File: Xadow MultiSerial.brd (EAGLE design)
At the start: 25.4 x 20.3 mm, 19 parts, among them J1 12p 0.5mm bottom contact, J2 12p 0.5mm bottom contact, J3 12p 0.5mm bottom contact, J4 12p 0.5mm bottom contact, U1 SC16IS752, X1 CTS_32X25_SMD

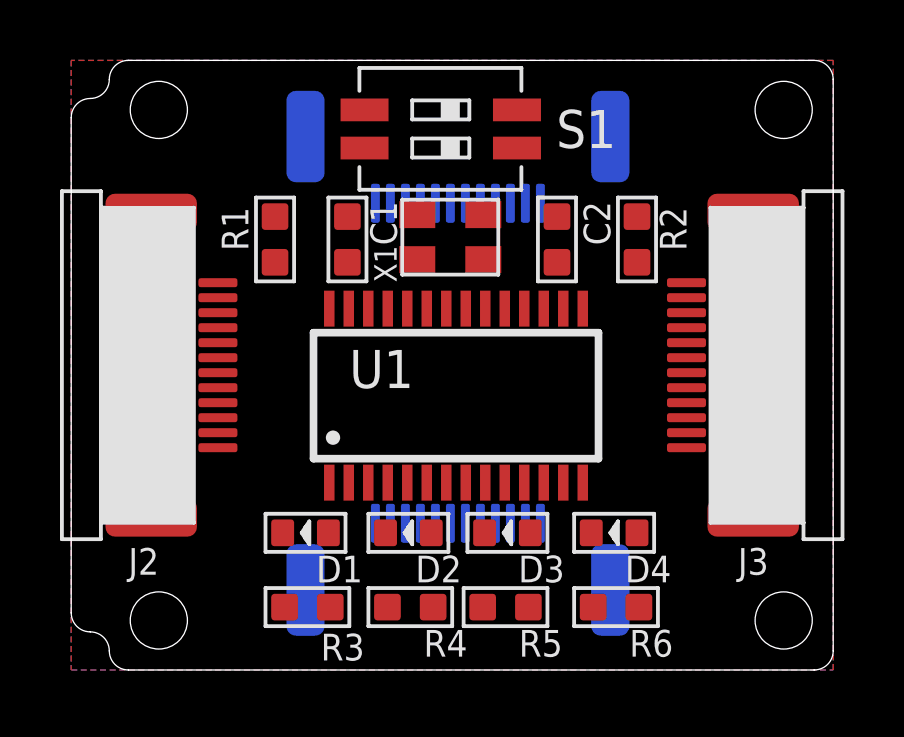
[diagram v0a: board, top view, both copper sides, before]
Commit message: Added level shifter MOSFETs
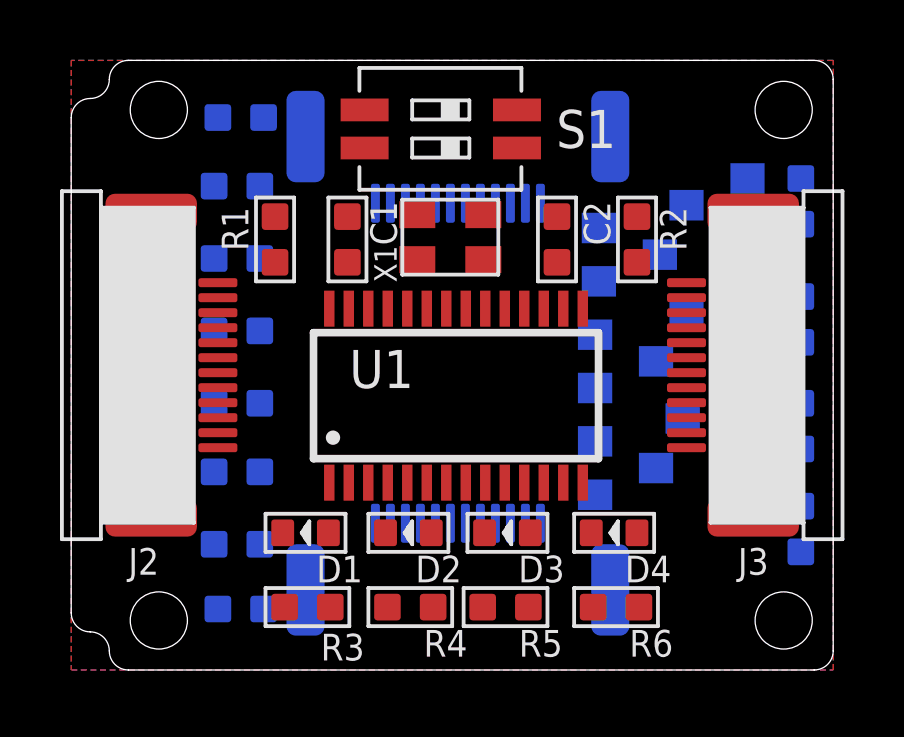
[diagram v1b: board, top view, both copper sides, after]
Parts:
- added Q1, Q2, Q3, Q4, Q5, Q6: MOSFET-N-044020001, OPL:SOT23
- added R10, R11, R12, R13, R14, R15, R16, R17, R18, R7, R8, R9: 10K, OPL:R0603
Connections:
- new net N$11: Q1.2, R7.1
- new net N$12: Q2.2, R9.1
- new net N$13: Q3.2, R11.1
- new net N$14: Q4.2, R13.1
- new net N$15: Q5.2, R15.1
- new net N$16: Q6.2, R17.1
- new net N$17: R10.2, R12.2, R14.2, R16.2, R18.2, R8.2
- new net N$18: Q1.3, R8.1
- new net N$19: Q2.3, R10.1
- new net N$20: Q3.3, R12.1
- new net N$21: Q4.3, R14.1
- new net N$22: Q5.3, R16.1
- new net N$23: Q6.3, R18.1
- new net N$4: Q1.1, Q2.1, Q3.1, Q4.1, Q5.1, Q6.1, R11.2, R13.2, R15.2, R17.2, R7.2, R9.2
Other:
- board text added: "Xadow Multiserial"
- board text added: "v1.0 14/09/2014"
- board text removed: "Breakout"
- board text removed: "Xadow"
- board text removed: "v1.0 03/19/2013"
